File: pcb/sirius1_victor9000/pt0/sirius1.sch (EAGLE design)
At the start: 28 parts, among them IC3 STM32F042F4, SW1 324_SW, SW4 324_SW, U1 RJ45

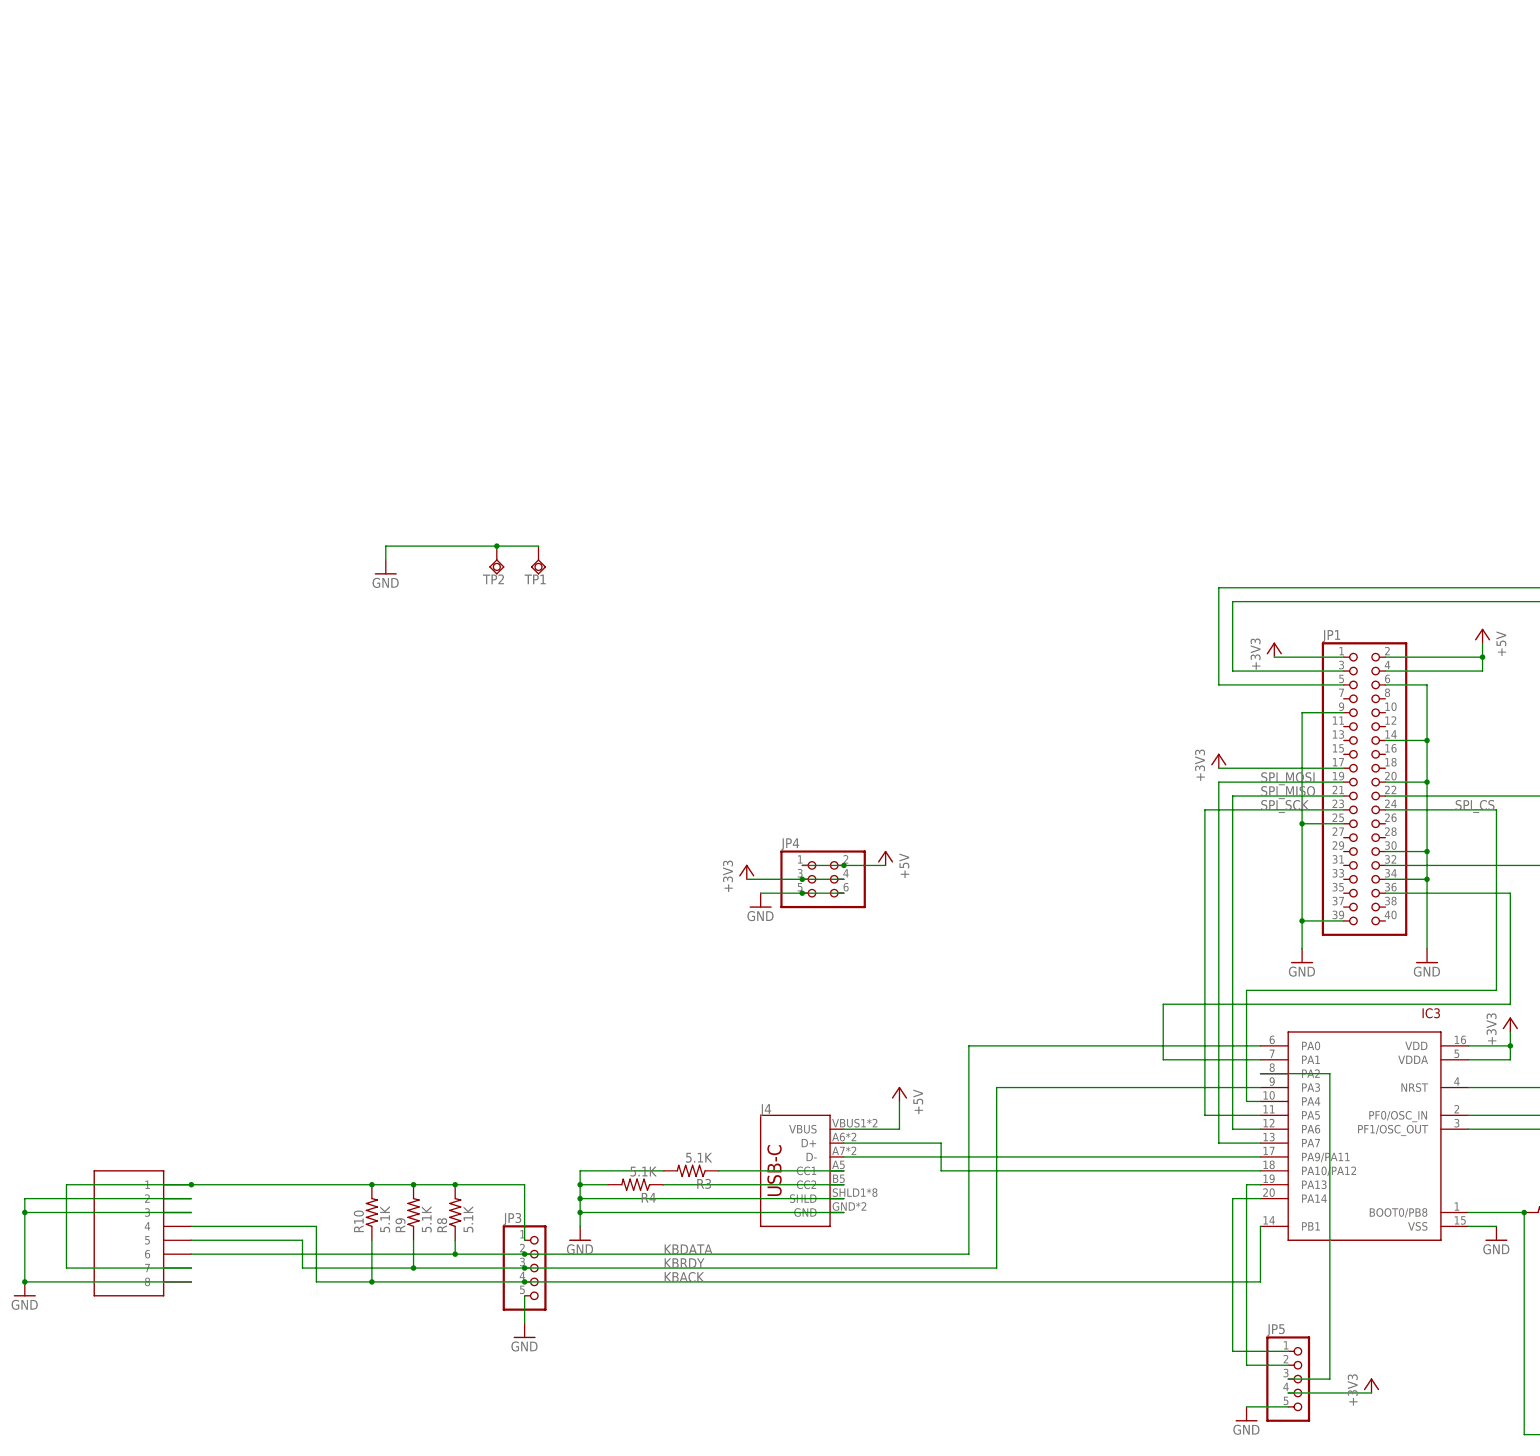
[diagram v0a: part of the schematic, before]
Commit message: updated sirius 1 pcb
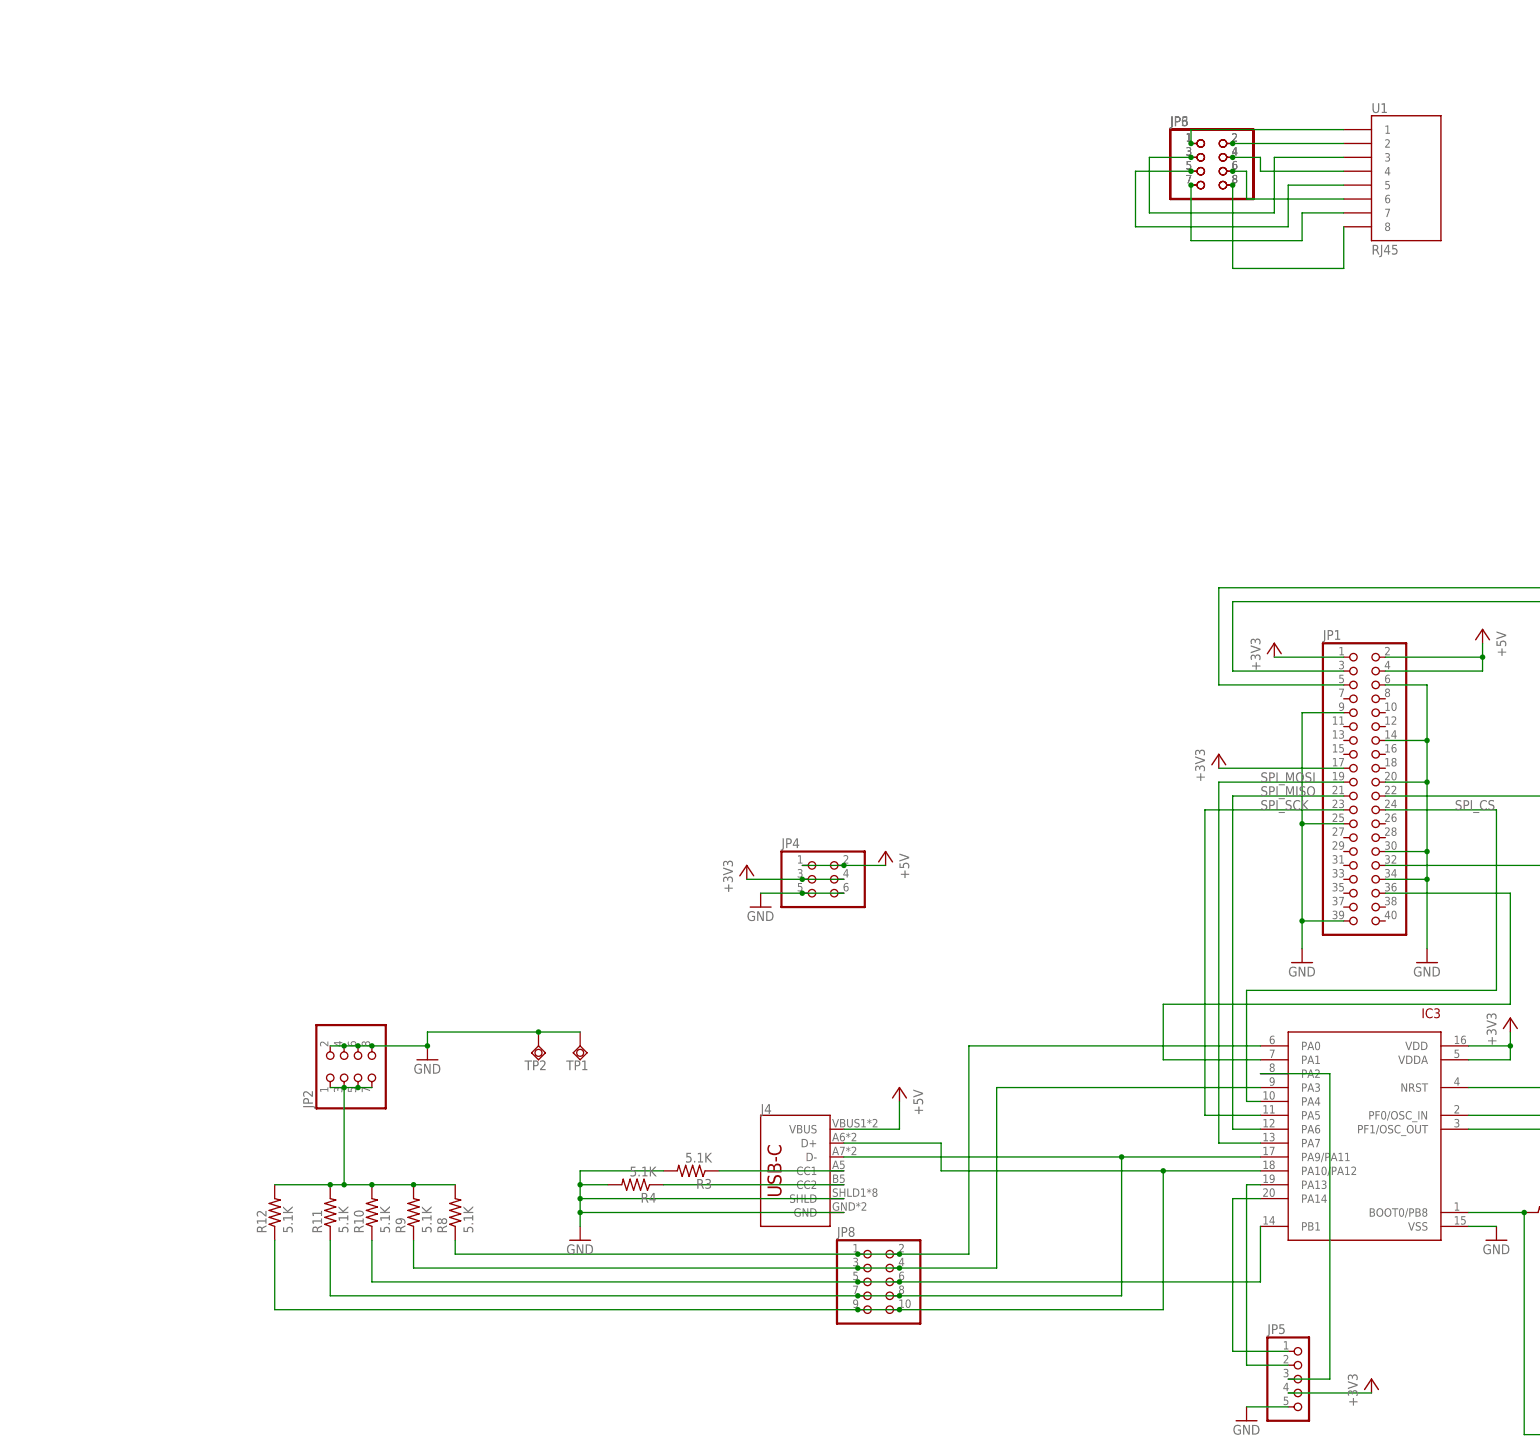
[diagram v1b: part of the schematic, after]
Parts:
- added JP2, JP6: (no value), pinhead:PINHD-2X4
- added JP8: (no value), pinhead:PINHD-2X5
- added R11, R12: 5.1K, SparkFun-Passives:RESISTOR0805-RES
- JP3: device pinhead:PINHD-1X5 -> pinhead:PINHD-2X4
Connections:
- removed net KBACK: IC3.PB1, JP3.4, R10.1, U1.4
- removed net KBDATA: IC3.PA0, JP3.2, R8.1, U1.6
- removed net KBRDY: IC3.PA3, JP3.3, R9.1, U1.5
- removed net N$3: IC3.PA9/PA11, J4.D-
- new net N$15: JP3.2, JP6.2, U1.2
- new net N$16: JP3.3, JP6.3, U1.3
- new net N$18: JP3.4, JP6.4, U1.4
- new net N$19: JP3.5, JP6.5, U1.5
- new net N$20: JP3.6, JP6.6, U1.6
- new net N$21: JP3.7, JP6.7, U1.7
- new net N$22: JP3.8, JP6.8, U1.8
- new net N$24: IC3.PA3, JP8.3, JP8.4, R9.1
- new net N$25: IC3.PB1, JP8.5, JP8.6, R10.1
- new net N$26: IC3.PA10/PA12, J4.D+, JP8.10, JP8.9, R12.1
- new net N$30: IC3.PA0, JP8.1, JP8.2, R8.1
- new net N$4: IC3.PA9/PA11, J4.D-, JP8.7, JP8.8, R11.1
- net GND: now also JP2.2, JP2.4, JP2.6, JP2.8; no longer JP3.5, U1.2, U1.3, U1.8
- net N$14: now also JP3.1, JP6.1, U1.1; no longer IC3.PA10/PA12, J4.D+
- net N$27: now also JP2.1, JP2.3, JP2.5, JP2.7, R11.2, R12.2; no longer JP3.1, U1.1, U1.7
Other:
- moved on the sheet: TP1, TP2
